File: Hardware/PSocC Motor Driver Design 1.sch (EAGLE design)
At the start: 43 parts, among them J1 DNP, J2 DNP, J3 DNP, J4 DNP, J5 DNP, J6 DNP, J7 DNP, U1 CY8C4245LQI-483, U2 DRV8835

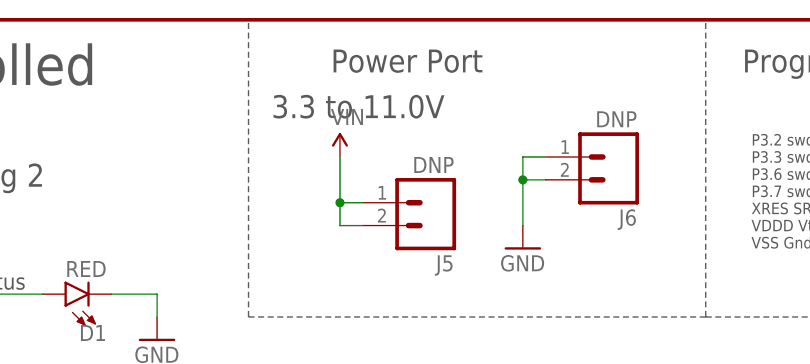
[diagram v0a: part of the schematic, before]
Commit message: Updated schematic docu
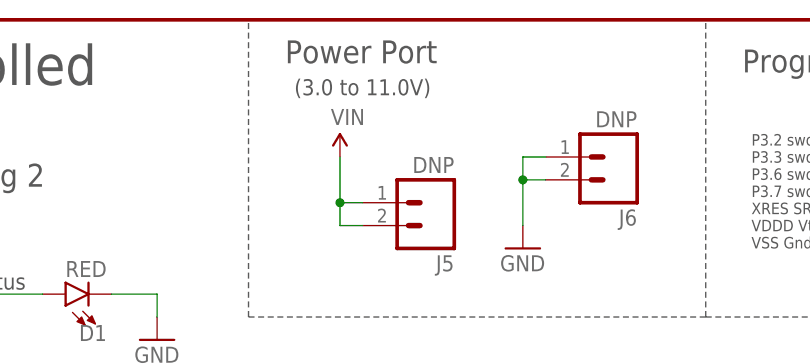
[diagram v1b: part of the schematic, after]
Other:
- note added: "(3.0 to 11.0V)"
- note removed: "3.3 to 11.0V"
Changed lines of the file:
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@@
 VSS Gnd</text>
 <text x="4.064" y="108.458" size="2.54" layer="97" font="vector" ratio="15">Serial Ports</text>
-<text x="75.184" y="179.578" size="2.54" layer="97" font="vector" ratio="15">Power Port</text>
+<text x="70.104" y="180.594" size="2.54" layer="97" font="vector" ratio="15">Power Port</text>
 <text x="120.904" y="179.578" size="2.54" layer="97" font="vector" ratio="15">Programming Header</text>
 <text x="95.504" y="108.458" size="2.54" layer="97" font="vector" ratio="15">H-Bridge Driver</text>
@@
 A '1' indicated solder bridge.</text>
 <text x="34.29" y="157.226" size="1.778" layer="97" font="vector" align="top-left">Status</text>
-<text x="68.58" y="177.038" size="2.54" layer="97" font="vector" ratio="15" align="top-left">3.3 to 11.0V</text>
+<text x="71.12" y="177.038" size="1.778" layer="97" font="vector" ratio="15">(3.0 to 11.0V)</text>
 </plain>
 <instances>
